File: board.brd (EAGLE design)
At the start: 107.9 x 68.3 mm, 77 parts, among them IC1 MC78M12BDTG, IC2 MC79M05CDTG, IC3 MC78M05CDTG, IC4 MC79M12BDTG, IC6 TPS77033, IC7 TPS77025, J1 XEM6310, U1 AD8022ARMZ, U2 AD5754BREZ, U3 ADR421ARMZ, X1 BU-SMA-V, X2 BU-SMA-V, X3 BU-SMA-V, X4 BU-SMA-V, X5 BU-SMA-V, X6 BU-SMA-V

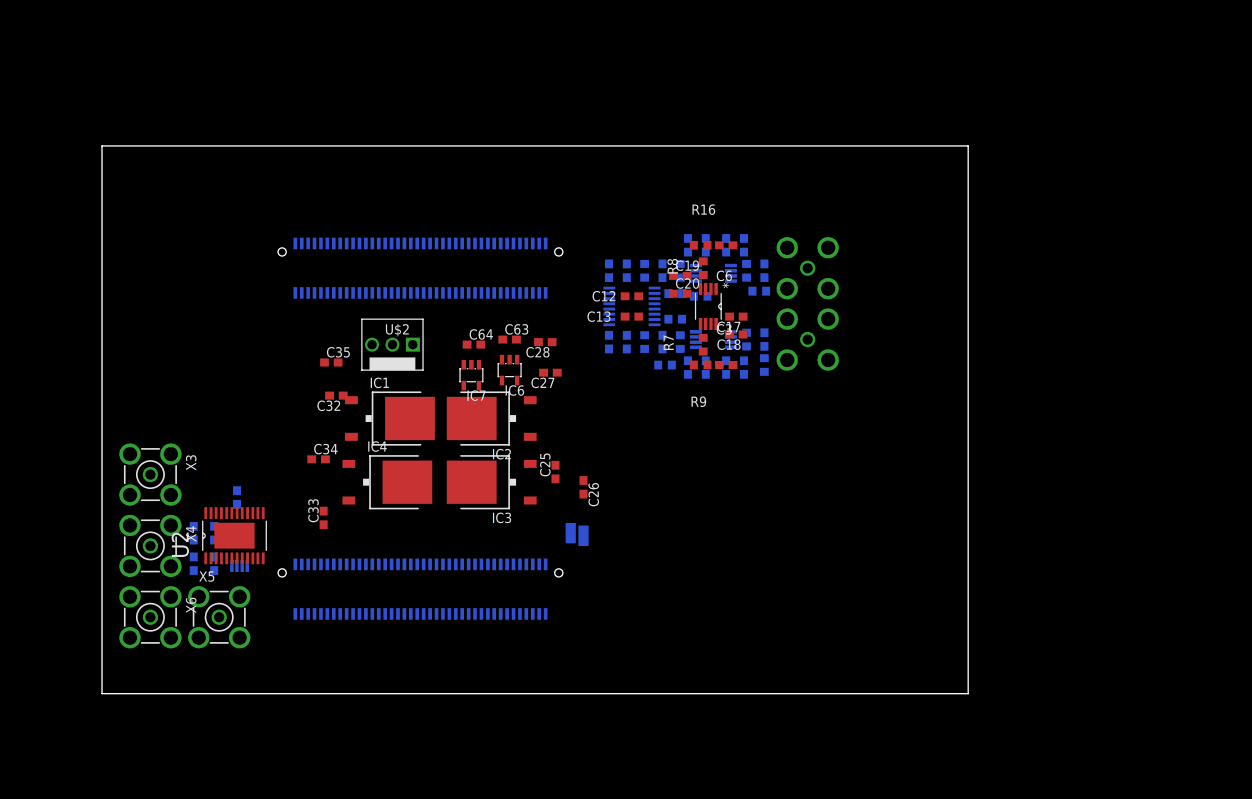
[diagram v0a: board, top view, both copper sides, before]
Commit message: Layout changes
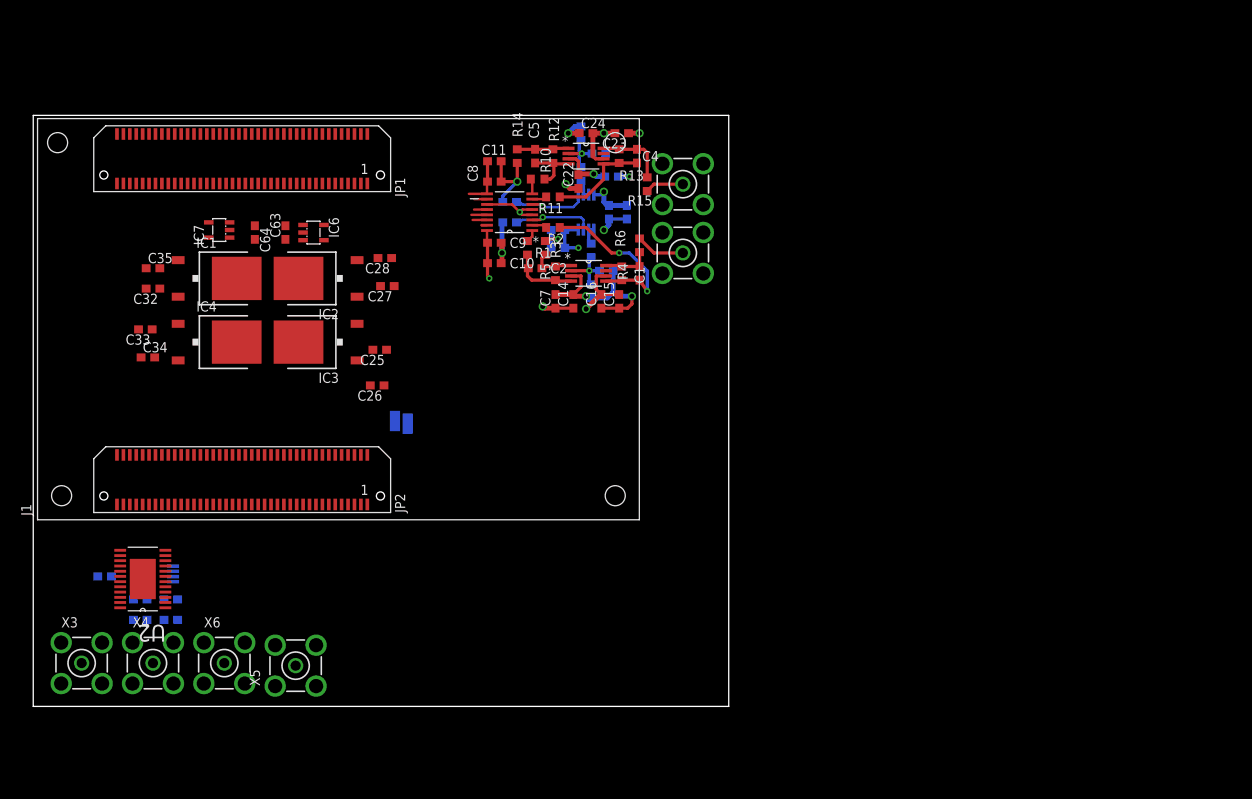
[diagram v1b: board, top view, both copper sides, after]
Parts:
- removed U$2: KK3V, molex-kk:KK-V-3
- moved IC7 36.3 mm to (23.2, 59.4), turned to 90 degrees
- moved C24 34.0 mm to (68.9, 71.4), flipped to the top, turned to 0 degrees
- moved C23 32.9 mm to (73.3, 71.4), flipped to the top, turned to 180 degrees
- moved R9 32.5 mm to (68.3, 71.4), flipped to the bottom, turned to 90 degrees
- moved C33 32.3 mm to (14.0, 47.0), turned to 180 degrees
- moved R14 31.9 mm to (60.3, 68.6), flipped to the top, turned to 90 degrees
- moved C63 31.0 mm to (31.4, 59.1), turned to 90 degrees
- moved C3 30.8 mm to (70.5, 68.9), flipped to the bottom, turned to 180 degrees
- moved C64 30.7 mm to (27.6, 59.1), turned to 270 degrees
- moved IC6 29.9 mm to (34.9, 59.1), turned to 270 degrees
- moved C26 28.7 mm to (42.9, 40.0), turned to 180 degrees
- moved C22 28.1 mm to (67.9, 65.4), flipped to the top
- moved C5 28.1 mm to (62.5, 68.6), flipped to the top, turned to 270 degrees
- moved R12 28.1 mm to (64.8, 68.6), flipped to the top, turned to 270 degrees
- moved ADCOP2 27.8 mm to (68.9, 68.6), flipped to the top, turned to 0 degrees
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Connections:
- net +15V: no longer U$2.1
- net -15V: no longer U$2.3
- net 0V: no longer U$2.2
- net GND: now also ADC1.12
- net GNDI: no longer ADC1.12
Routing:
- net GND: track 0.00 -> 60.1 mm, vias 0 -> 11
- net +5V: track 0.00 -> 56.6 mm, vias 0 -> 3
- net -5V: track 0.00 -> 53.6 mm, vias 0 -> 3
- net N$2: track 0.00 -> 21.6 mm, vias 0 -> 2
- net N$14: track 0.00 -> 12.7 mm
- net VREF1A: track 0.00 -> 11.4 mm, vias 0 -> 1
- net VREF1B: track 0.00 -> 10.6 mm, vias 0 -> 1
- net N$16: track 0.00 -> 8.72 mm
- net N$12: track 0.00 -> 8.43 mm
- net N$9: track 0.00 -> 7.70 mm, vias 0 -> 1
- net +3V3: track 0.00 -> 7.35 mm, vias 0 -> 1
- net N$20: track 0.00 -> 7.02 mm
- net N$17: track 0.00 -> 6.96 mm, vias 0 -> 1
- net N$15: track 0.00 -> 6.44 mm
- net VDD: track 0.00 -> 6.35 mm
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- added copper zone on layer 2, net GND
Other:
- board size 107.9 x 68.3 mm -> 86.7 x 73.7 mm

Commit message: Back to latest revision
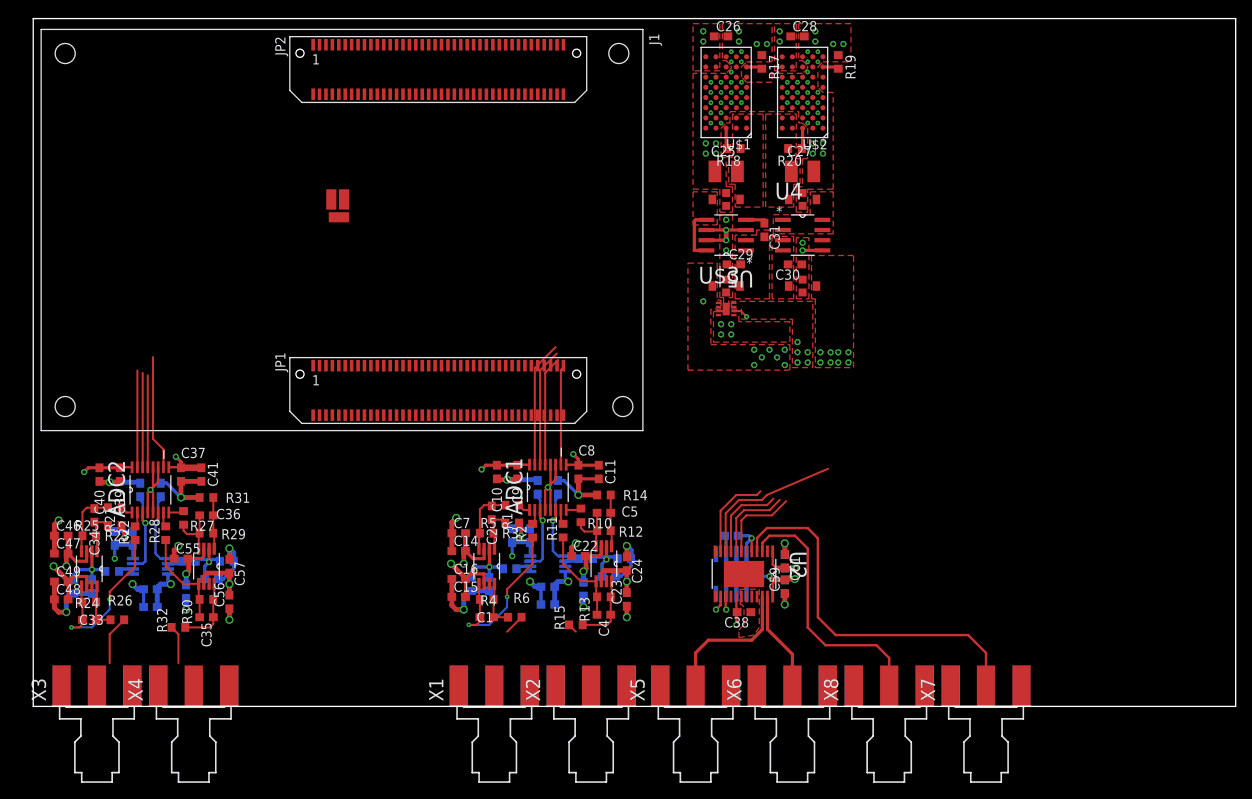
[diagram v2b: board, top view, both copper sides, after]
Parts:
- removed C63, C64: 4.7uF, rcl:C0603
- removed IC1: MC78M12BDTG, linear:DPACK_3
- removed IC2: MC79M05CDTG, linear:DPACK_3
- removed IC3: MC78M05CDTG, linear:DPACK_3
- removed IC4: MC79M12BDTG, linear:DPACK_3
- removed IC6: TPS77033, texas:SOT23-DBV
- removed IC7: TPS77025, texas:SOT23-DBV
- added ADC2: AD7357BRUZ, Analog Devices_By_element14_Batch_1:SOP65P640X120-16N
- added ADCOP3, ADCOP4: AD8138ARMZ, Analog Devices_By_element14_Batch_1:SOP65P490X110-8N
- added C29, C37, C39, C42, C43, C46, C48, C50, C52, C54, C56: 10uF, rcl:C0603
- added C30: 0.1uF Tant, rcl:C0603
- added C31: 0.01uF, rcl:C0603
- added C36: 39pF, rcl:C0603
- added C40, C41, C44, C45, C47, C49, C51, C53, C55, C57: 0.1uF, rcl:C0603
- added R17: 115k, resistor:R0603
- added R18: 51k, resistor:R0603
- added R19: 130k, resistor:R0603
- added R20: 66k, resistor:R0603
- added R21, R22, R27, R28: 33, resistor:R0603
- added R23, R24, R25, R26, R29, R30, R31, R32: 499, resistor:R0603
- added R33, R34, R35, R36: 10K, resistor:R0603
- added SH3: SHORT-HB5, shorts:SHORT_BOT-50
- added U$1, U$2: LTM8045, adc:BGA-40
- added U$3: ADP222ACPZ-3325-R7, ADI-Phase-2:QFN50P200X200X60-9N
- added U$4, U$5, U$6, U$7: NFM31P, adc:NFM31P
- added U4: LT1175CS8-5PBF, LTC_By_element14_Batch_1:SOIC127P600X175-8N
- added U5: LT1763CS8-5PBF, LTC_By_element14_Batch_1:SOIC127P600X175-8N
- added U6: AD8022ARMZ, Analog Devices_By_element14_Batch_1:SOP65P490X110-8N
- added X7, X8: SMA-142-0701-871/876, con-coax:J502-ND-142-0701-871/876
- C25: value 10uF -> 100uF; device rcl:C0603 -> rcl:C1210
- C26: value 0.1uF -> 4.7uF
- C27: value 0.1uF -> 100uF; device rcl:C0603 -> rcl:C1210
- C28: value 10uF -> 4.7uF
- C33, C34: value 10uF -> 39pF
- C35: value 0.1uF -> 39pF
- J1: device opalkelly:XEM6310 -> adc:XEM6310
- U3: value ADR421ARMZ -> ADR420ARZ; device ADI-Phase-2:SOP65P490X110-8N -> Analog Devices_By_element14_Batch_1:SOIC127P600X175-8N
- X1, X2, X3, X4, X5, X6: value BU-SMA-V -> SMA-142-0701-871/876; device con-coax:BU-SMA-V -> con-coax:J502-ND-142-0701-871/876
- moved C59 80.4 mm to (93.7, 14.9), flipped to the top, turned to 90 degrees
- moved C58 80.3 mm to (93.7, 14.9), turned to 90 degrees
- moved C38 79.8 mm to (88.6, 11.7), flipped to the top
- moved C32 78.4 mm to (87.0, 21.3), flipped to the bottom
- moved C60 76.9 mm to (93.7, 18.1), turned to 270 degrees
- moved C61 76.7 mm to (93.7, 18.1), flipped to the top, turned to 270 degrees
- moved U2 74.9 mm to (88.6, 16.5), turned to 270 degrees
- moved U3 71.8 mm to (87.0, 16.5), turned to 270 degrees
- moved X6 71.0 mm to (94.6, 0.00), turned to 90 degrees
- moved X2 66.1 mm to (69.5, 0.00), turned to 90 degrees
- moved X1 61.2 mm to (57.5, 0.00)
- moved C26 61.1 mm to (85.7, 83.5), turned to 0 degrees
- moved C28 58.4 mm to (95.2, 83.5), turned to 0 degrees
- moved C23 58.1 mm to (74.0, 13.3), turned to 90 degrees
- moved C4 57.3 mm to (71.1, 11.4), turned to 180 degrees
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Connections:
- removed net +12V: C33.2, C58.2, C59.2, IC1.3, U2.24, U3.2
- removed net +15V: C26.2, C32.2, IC1.1, IC3.1
- removed net -12V: C34.2, C60.2, C61.2, IC4.3, U2.1
- removed net -15V: C27.2, C35.2, IC2.4, IC4.4
- new net ADC10: ADC2.10
- new net ADC11: ADC2.13
- new net ADC12: ADC2.14
- new net ADC13: ADC2.15
- new net GNDINT: C29.1, C30.1, SH1.1, SH2.1, SH3.1, U$3.3, U$3.9, U$6.GND, U$6.GND2, U$7.GND, U$7.GND2, U4.5, U5.3, U5.6, U5.7
- new net N$23: ADCOP3.5, C33.2, R22.1, R24.2
- new net N$26: ADCOP3.1, C34.1, R23.1, R25.2
- new net N$27: U$2.G3
- new net N$28: ADCOP3.8, C33.1, R24.1, R26.2
- new net N$29: U$1.G3
- new net N$30: R19.2, U$2.G1
- new net N$32: R17.2, U$1.G1
- new net N$33: U$2.E1
- new net N$34: R18.2, U$1.A3
- new net N$35: C25.2, R18.1, U$1.A1, U$1.A2, U$1.B1, U$1.B2, U$4.IN
- new net N$36: ADC2.1, R21.2
- new net N$37: C27.1, R20.2, U$2.A4, U$2.A5, U$2.B4, U$2.B5, U$5.IN
- new net N$38: R20.1, U$2.A3
- new net N$39: ADC2.2, R22.2
- new net N$40: ADCOP3.4, C34.2, R21.1, R23.2
- new net N$41: ADCOP4.5, C35.2, R28.1, R30.2
- new net N$42: ADCOP4.1, C36.1, R29.1, R31.2
- new net N$43: ADCOP4.8, C35.1, R30.1, R32.2
- new net N$44: ADCOP4.4, C36.2, R27.1, R29.2
- new net N$45: ADC2.8, R27.2
- new net N$46: ADC2.7, R28.2
- new net N$47: R32.1, X4.1
- new net N$48: U$5.OUT, U4.1, U4.2, U4.7, U4.8
- new net N$49: C31.1, U5.4
- new net N$51: R26.1, X3.1
- new net N$52: R33.1, U6.6, U6.7
- new net N$54: R34.1, U6.1, U6.2
- new net N$57: ADCOP3.2, C45.2, R34.2, R36.2
- new net N$59: ADCOP4.2, C44.1, R33.2, R35.1
- new net N$65: U$4.OUT, U5.5, U5.8
- new net N$66: C30.2, U$6.IN, U4.3, U4.4
- new net N$67: C29.2, C31.2, U$7.IN, U5.1, U5.2
- new net V+: C26.1, C28.1, U$1.G4, U$1.G5, U$1.H4, U$1.H5, U$2.G4, U$2.G5, U$2.H4, U$2.H5
- new net VREF2A: ADC2.3, C42.1, U6.3
- new net VREF2B: ADC2.6, C43.1, U6.5
- net +3V3: now also ADC2.16, C39.1, C40.1, U$3.7, U$3.8; no longer IC6.5
- net +5V: now also ADCOP3.3, ADCOP4.3, C32.1, C46.2, C47.2, C50.2, C51.2, C54.2, C55.2, C58.2, C59.2, U$3.1, U$3.2, U$3.6, U$7.OUT, U2.24, U3.2, U6.8; no longer C25.2, C63.2, C64.2, IC3.3, IC6.1, IC7.1
- net -5V: now also ADCOP3.6, ADCOP4.6, C48.2, C49.2, C52.2, C53.2, C56.2, C57.2, C60.2, C61.2, U$6.OUT, U2.1, U6.4; no longer C28.2, IC2.3
- net 0V: now also C26.2, C27.2, C28.2, R17.1, R19.1, SH1.2, U$1.A4, U$1.A5, U$1.B3, U$1.B4, U$1.B5, U$1.C1, U$1.C2, U$1.C3, U$1.C4, U$1.C5, U$1.D1, U$1.D2, U$1.D3, U$1.D4, U$1.D5, U$1.E1, U$1.E2, U$1.E3, U$1.E4, U$1.E5, U$1.F2, U$1.F3, U$1.F4, U$1.F5, U$1.G2, U$1.H1, U$1.H2, U$1.H3, U$2.A1, U$2.A2, U$2.B1, U$2.B2, U$2.B3, U$2.C1, U$2.C2, U$2.C3, U$2.C4, U$2.C5, U$2.D1, U$2.D2, U$2.D3, U$2.D4, U$2.D5, U$2.E2, U$2.E3, U$2.E4, U$2.E5, U$2.F2, U$2.F3, U$2.F4, U$2.F5, U$2.G2, U$2.H1, U$2.H2, U$2.H3, U$4.GND, U$4.GND2, U$5.GND, U$5.GND2; no longer C26.1, C27.1, C28.1, C32.1, C33.1, C34.1, C35.1, C63.1, C64.1, IC1.4, IC2.1, IC3.4, IC4.1, IC6.2, IC6.3, IC7.2, IC7.3, SH2.2
- net ADC0: now also ADC1.10, J1.170; no longer ADC1.15, J1.224
- net ADC1: now also ADC1.13, J1.168; no longer ADC1.10, J1.223
- net ADC2: now also J1.166; no longer J1.222
- net ADC3: now also ADC1.15, J1.164; no longer ADC1.13, J1.221
- net ADC4: now also J1.172; no longer J1.225
- net ADC5: now also J1.174; no longer J1.226
- net ADC6: now also J1.176; no longer J1.227
- net DACD0: now also J1.224; no longer J1.215
- net DACD1: now also J1.222; no longer J1.216
- net DACD2: now also J1.218; no longer J1.217
- net DACD3: now also J1.220; no longer J1.218
- net DACD4: now also J1.216; no longer J1.219
- net GND: now also ADC2.11, ADC2.12, ADC2.4, ADC2.5, C32.2, C37.2, C39.2, C40.2, C41.2, C42.2, C43.2, C44.2, C45.1, C46.1, C47.1, C48.1, C49.1, C50.1, C51.1, C52.1, C53.1, C54.1, C55.1, C56.1, C57.1, R25.1, R31.1, R35.2, R36.1, SH3.2, X1.G@1, X1.G@2, X1.G@3, X1.G@4, X2.G@1, X2.G@2, X2.G@3, X2.G@4, X3.G@1, X3.G@2, X3.G@3, X3.G@4, X4.G@1, X4.G@2, X4.G@3, X4.G@4, X5.G@1, X5.G@2, X5.G@3, X5.G@4, X6.G@1, X6.G@2, X6.G@3, X6.G@4, X7.G@1, X7.G@2, X7.G@3, X7.G@4, X8.G@1, X8.G@2, X8.G@3, X8.G@4; no longer SH1.2, SH2.1, X1.2, X1.3, X1.4, X1.5, X2.2, X2.3, X2.4, X2.5, X3.2, X3.3, X3.4, X3.5, X4.2, X4.3, X4.4, X4.5, X5.2, X5.3, X5.4, X5.5, X6.2, X6.3, X6.4, X6.5
- net GNDI: now also SH2.2; no longer SH1.1
- net N$18: now also X7.1; no longer X5.1
- net N$19: now also X6.1; no longer X4.1
- net N$21: now also X8.1; no longer X6.1
- net N$5: now also X5.1; no longer X3.1
- net VDD: now also ADC2.9, C37.1, C41.1, U$3.4, U$3.5; no longer IC7.5
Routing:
- net GND: track 60.1 -> 139.4 mm, vias 11 -> 26
- net N$18: track 0.00 -> 47.0 mm
- net N$21: track 0.00 -> 32.8 mm
- net N$23: track 0.00 -> 22.0 mm, vias 0 -> 2
- net DACD2: track 0.00 -> 19.1 mm
- net N$5: track 0.00 -> 17.7 mm
- net N$19: track 0.00 -> 15.3 mm
- net ADC10: track 0.00 -> 14.3 mm
- net ADC3: track 1.96 -> 15.7 mm
- net ADC2: track 1.80 -> 14.7 mm
- net N$41: track 0.00 -> 12.7 mm
- net GNDINT: track 0.00 -> 12.3 mm, vias 0 -> 6
- net ADC1: track 1.59 -> 13.7 mm
- net ADC13: track 0.00 -> 12.1 mm
- net ADC12: track 0.00 -> 11.8 mm
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- added copper zone on layer 1, net +3V3
- added copper zone on layer 15, net +3V3
- added copper zone on layer 1, net +5V
- added copper zone on layer 15, net +5V
- added copper zone on layer 1, net -5V
- added copper zone on layer 15, net -5V
- added copper zone on layer 1, net 0V
- added copper zone on layer 2, net 0V
- added copper zone on layer 1, net GND
- added copper zone on layer 1, net GNDINT
- added copper zone on layer 2, net GNDINT
- added copper zone on layer 1, net N$35
- added copper zone on layer 1, net N$37
- added copper zone on layer 1, net N$48
- added copper zone on layer 1, net N$65
- added copper zone on layer 1, net N$66
- added copper zone on layer 1, net N$67
- added copper zone on layer 1, net V+
- added copper zone on layer 1, net VDD
- added copper zone on layer 15, net VDD
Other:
- board size 86.7 x 73.7 mm -> 149.9 x 85.7 mm
- board text removed: "1"
- board text removed: "2A"
- board text removed: "2B"
- board text removed: "EXT"
